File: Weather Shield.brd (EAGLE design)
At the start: 53.3 x 59.7 mm, 46 parts, among them J1 GP-635T, Q1 BSS138, Q2 BSS138, U1 ARDUINO_R3_SHIELD, U2 3.3V MIC5219, U3 ALS-PT19, U4 MPL3115A2LGA8, U5 HTU21D

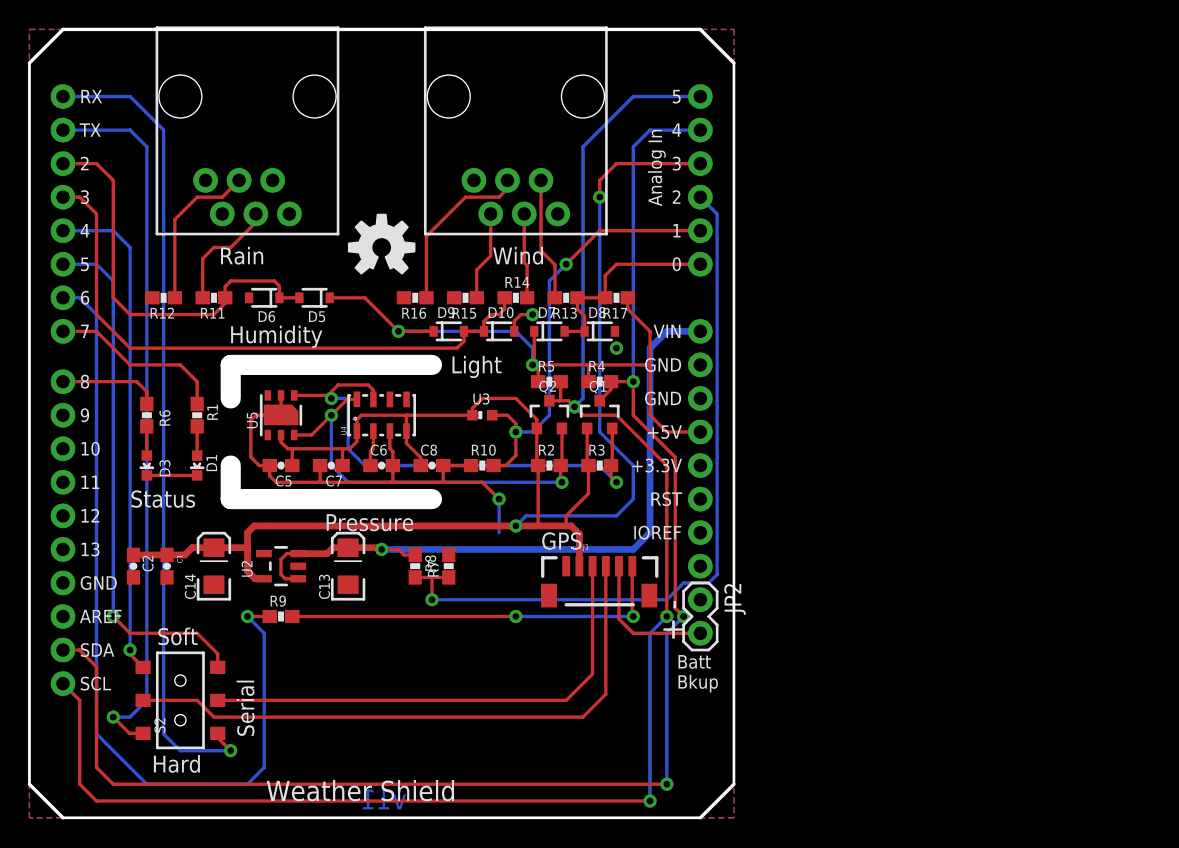
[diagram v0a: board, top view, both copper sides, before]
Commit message: Initial commit
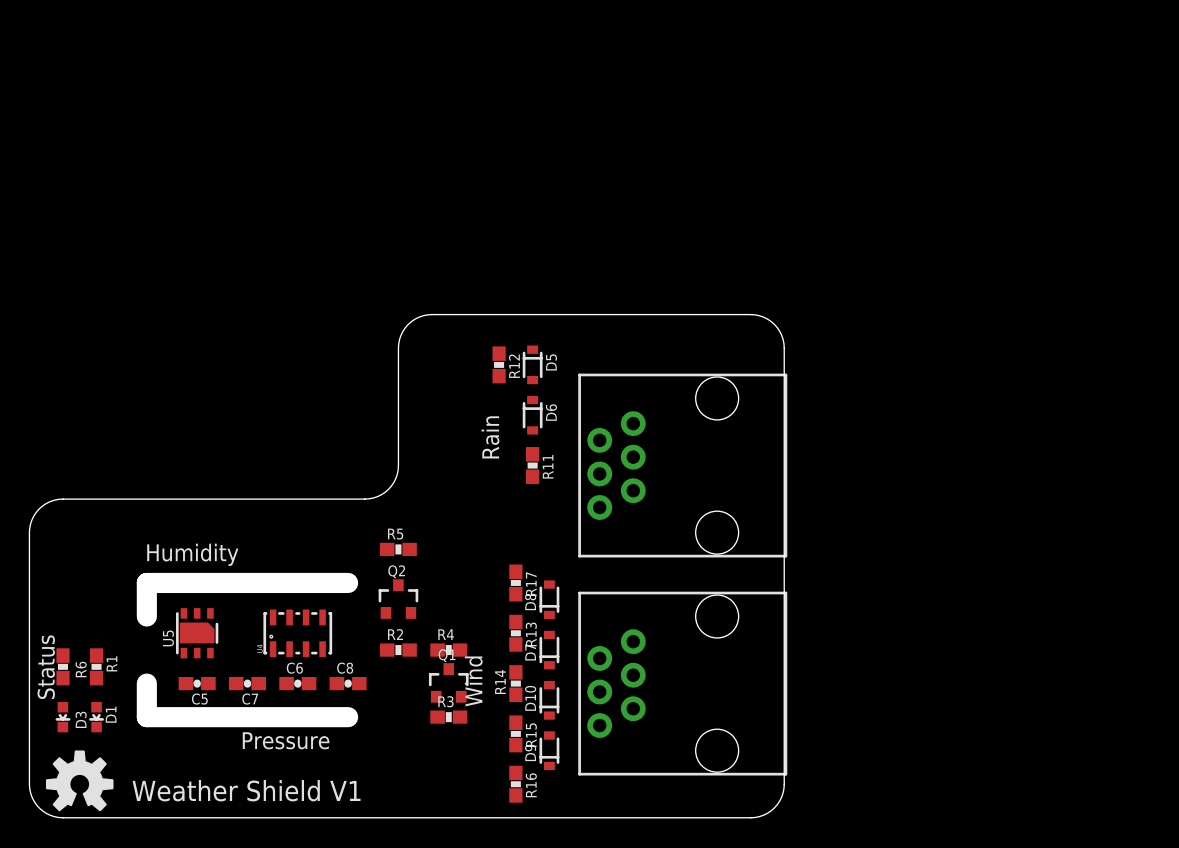
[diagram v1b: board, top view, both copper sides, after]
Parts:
- removed C1: 1uF, SparkFun:0603-CAP
- removed C13, C14: 10uF, SparkFun-Passives:EIA3216
- removed C2: 0.1uF, SparkFun:0603-CAP
- removed J1: GP-635T, SparkFun-Sensors:GP-635T
- removed JP2: External Batt Bckup, SparkFun-Connectors:1X02
- removed R10: 10K, SparkFun-Passives:0603-RES
- removed R7: 1K, SparkFun:0603-RES
- removed R8: 3.9K, SparkFun:0603-RES
- removed R9: 4.7K, SparkFun:0603-RES
- removed S2: Serial Select, SparkFun-Electromechanical:AYZ0202
- removed U1: ARDUINO_R3_SHIELD, SparkFun-Boards:UNO_R3_SHIELD
- removed U2: 3.3V MIC5219, SparkFun:SOT23-5
- removed U3: ALS-PT19, SparkFun-Sensors:ALS-PT19
- D1: value Blue -> Red
- moved JP10-DNP 50.6 mm to (52.1, 5.08), turned to 90 degrees
- moved LOGO1 46.6 mm to (3.81, 2.54)
- moved JP9-DNP 44.9 mm to (52.1, 21.6), turned to 90 degrees
- moved R16 37.6 mm to (36.8, 2.54), turned to 270 degrees
- moved R15 33.2 mm to (36.8, 6.35), turned to 270 degrees
- moved D9 32.7 mm to (39.4, 5.08), turned to 90 degrees
- moved R14 29.2 mm to (36.8, 10.2), turned to 90 degrees
- moved D10 28.2 mm to (39.4, 8.89), turned to 90 degrees
- moved R11 27.3 mm to (38.1, 26.7), turned to 270 degrees
- moved R12 25.9 mm to (35.6, 34.3), turned to 270 degrees
- moved R13 25.7 mm to (36.8, 14.0), turned to 270 degrees
- moved D7 24.1 mm to (39.4, 12.7), turned to 90 degrees
- moved R4 23.3 mm to (31.8, 12.7)
- moved Q1 23.3 mm to (31.8, 10.2)
- moved R17 22.9 mm to (36.8, 17.8), turned to 270 degrees
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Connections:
- removed net 3V_PWR_CTL: J1.6, R9.2
- removed net BATT_LVL: R7.1, R8.2, U1.A2
- removed net GPS-RX: J1.4, S2.2
- removed net GPS-TX: J1.3, S2.5
- removed net GRXI: S2.6, U1.D5
- removed net GTXO: S2.3, U1.D4
- removed net LIGHT: R10.2, U1.A1, U3.E
- removed net PWR_CTL: R9.1, U1.D6
- removed net RAW: C13.A, R8.1, U1.VIN, U2.1, U2.3
- removed net RXI: S2.4, U1.RX
- removed net TXO: S2.1, U1.TX
- removed net V_BATT: J1.5, JP2.2
- net 3.3V: no longer C1.1, C14.A, C2.1, J1.2, U1.A3, U2.5, U3.C
- net 5V: no longer U1.5V
- net GND: no longer C1.2, C13.C, C14.C, C2.2, J1.1, JP2.1, R10.1, R7.2, U1.GND@0, U1.GND@1, U1.GND@2, U2.2
- net HV_SCL: no longer U1.A5, U1.SCL
- net HV_SDA: no longer U1.A4, U1.SDA
- net RAIN: no longer U1.D2
- net STAT1: no longer U1.D7
- net STAT2: no longer U1.D8
- net WDIR: no longer U1.A0
- net WSPEED: no longer U1.D3
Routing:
- net 3.3V: track 131.2 -> 0.00 mm, vias 2 -> 0
- net HV_SCL: track 120.6 -> 0.00 mm, vias 3 -> 0
- net HV_SDA: track 113.8 -> 0.00 mm, vias 3 -> 0
- net PWR_CTL: track 63.3 -> 0.00 mm, vias 1 -> 0
- net RXI: track 61.7 -> 0.00 mm, vias 1 -> 0
- net BATT_LVL: track 55.7 -> 0.00 mm, vias 1 -> 0
- net TXO: track 54.6 -> 0.00 mm, vias 1 -> 0
- net RAW: track 52.5 -> 0.00 mm, vias 1 -> 0
- net 5V: track 49.1 -> 0.00 mm, vias 2 -> 0
- net GPS-RX: track 46.0 -> 0.00 mm
- net WSPEED: track 45.6 -> 0.00 mm
- net GND: track 44.7 -> 0.00 mm, vias 3 -> 0
- net GRXI: track 39.8 -> 0.00 mm, vias 1 -> 0
- net SDA: track 38.4 -> 0.00 mm, vias 2 -> 0
- net GTXO: track 37.8 -> 0.00 mm, vias 1 -> 0
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- removed copper zone on layer 1, net GND
- removed copper zone on layer 16, net GND
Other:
- board size 53.3 x 59.7 mm -> 57.1 x 38.1 mm
- board text added: "Weather Shield V1"
- board text removed: "+"
- board text removed: "-"
- board text removed: "Batt Bkup"
- board text removed: "GPS"
- board text removed: "Hard"
- board text removed: "Light"
- board text removed: "Serial"
- board text removed: "Soft"
- board text removed: "Weather Shield"
- board text removed: "v11"

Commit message: Initial commit
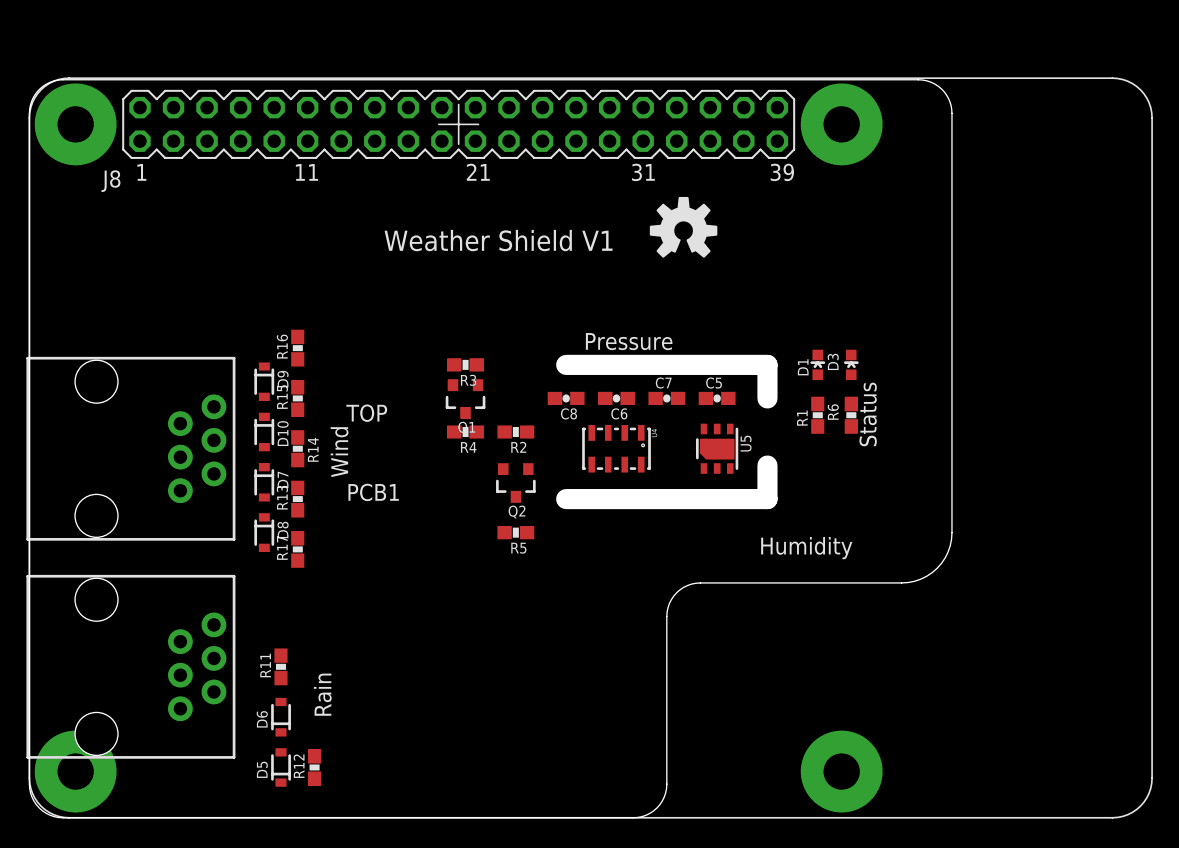
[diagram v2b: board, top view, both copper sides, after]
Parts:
- added PCB1: RASPBERRY_PI_B+_TPLACE, RASPBERRY_PI_Bplus:RASPBERRY_PI_BPLUS_TPLACE
- moved D3 65.4 mm to (62.2, 34.3), turned to 0 degrees
- moved R6 62.7 mm to (62.2, 30.5), turned to 90 degrees
- moved LOGO1 62.0 mm to (49.5, 44.5)
- moved D1 60.8 mm to (59.7, 34.3), turned to 0 degrees
- moved R1 57.8 mm to (59.7, 30.5), turned to 90 degrees
- moved JP10-DNP 54.7 mm to (5.08, 33.0), turned to 270 degrees
- moved JP9-DNP 47.3 mm to (5.08, 16.5), turned to 270 degrees
- moved C5 44.9 mm to (52.1, 31.8), turned to 0 degrees
- moved U5 41.8 mm to (52.1, 27.9), turned to 270 degrees
- moved C7 38.4 mm to (48.3, 31.8), turned to 0 degrees
- moved R16 36.9 mm to (20.3, 35.6), turned to 90 degrees
- moved D5 35.9 mm to (19.1, 3.81), turned to 90 degrees
- moved D9 35.3 mm to (17.8, 33.0), turned to 270 degrees
- moved R12 33.5 mm to (21.6, 3.81), turned to 90 degrees
- moved C6 32.4 mm to (44.5, 31.8), turned to 180 degrees
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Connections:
- new net 3V3: PCB1.1, PCB1.17
- new net 5V0: PCB1.2, PCB1.4
- net GND: now also PCB1.14, PCB1.20, PCB1.25, PCB1.30, PCB1.34, PCB1.39, PCB1.6, PCB1.9
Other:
- board size 57.1 x 38.1 mm -> 69.8 x 55.9 mm
